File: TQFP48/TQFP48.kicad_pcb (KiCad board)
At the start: 2 copper layers, 61.2 x 18 mm, 11 parts, among them J1 Conn_01x24, J2 Conn_02x24_Counter_Clockwise, J3 Conn_02x24_Counter_Clockwise, J4 Conn_01x24, J5 Conn_01x05

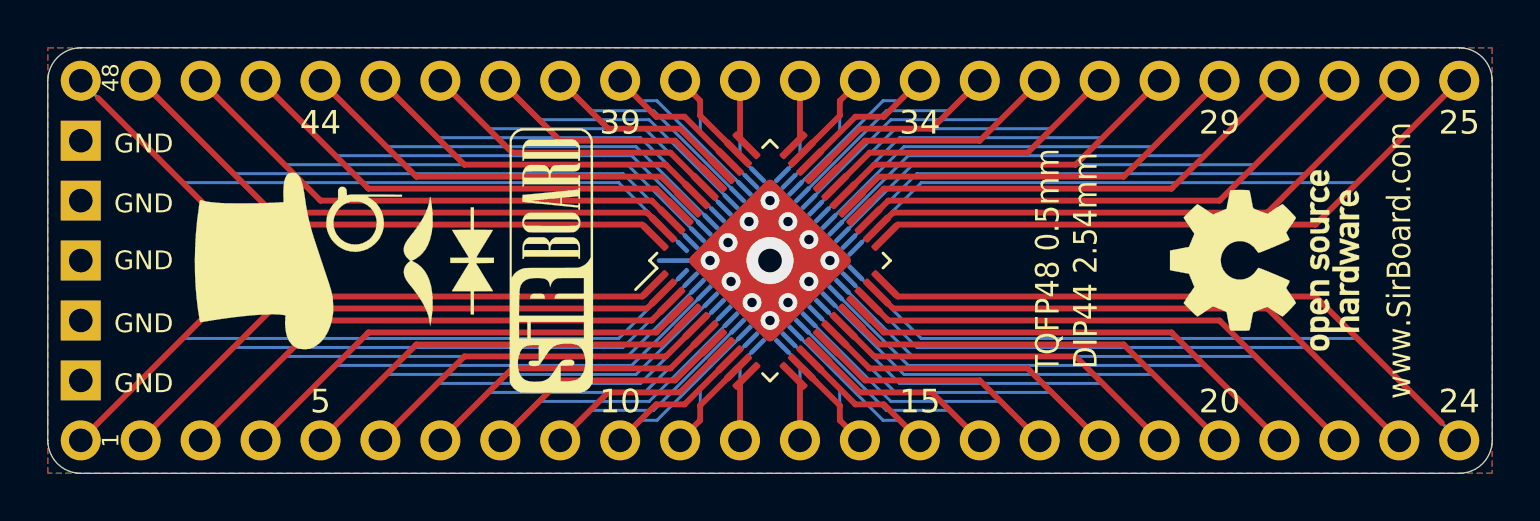
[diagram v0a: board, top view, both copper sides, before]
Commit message: Board Updates
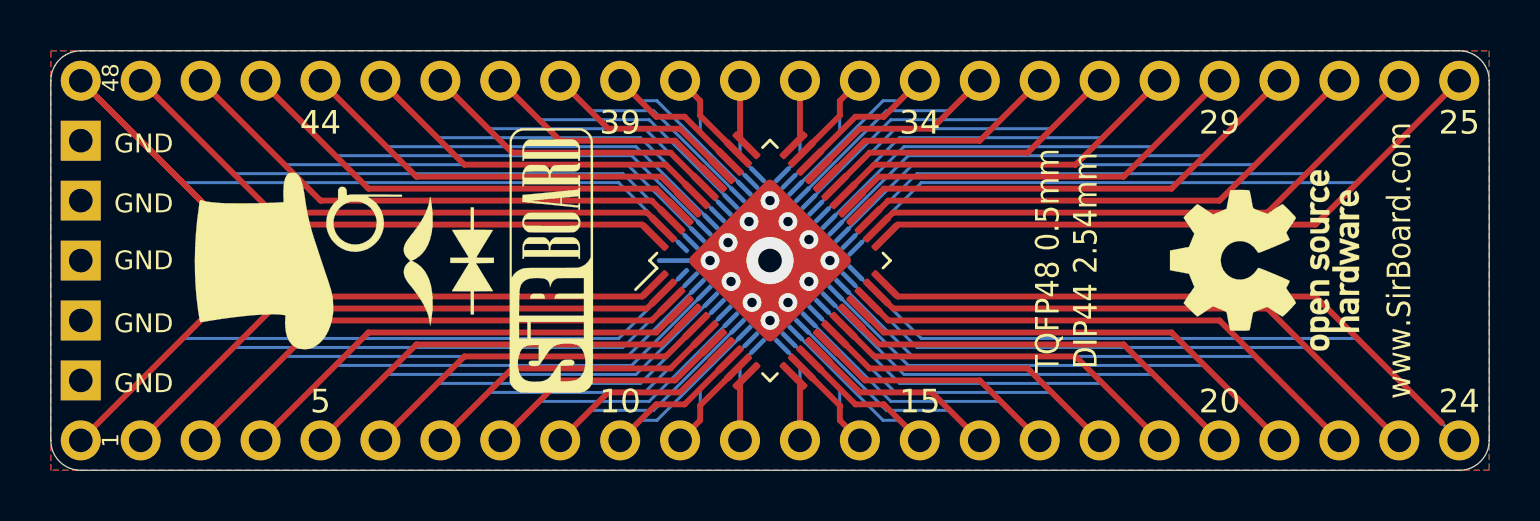
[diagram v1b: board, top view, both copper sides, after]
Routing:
- net Net-(J2-Pad48): track 54.5 -> 62.1 mm
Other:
- board size 61.2 x 18 mm -> 61 x 17.8 mm
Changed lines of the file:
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@@
     (thickness 1.6)
     (drawings 76)
-    (tracks 326)
+    (tracks 327)
     (zones 0)
     (modules 11)
@@
     (38 B.Mask user hide)
     (39 F.Mask user hide)
-    (40 Dwgs.User user)
+    (40 Dwgs.User user hide)
     (41 Cmts.User user hide)
     (42 Eco1.User user hide)
@@
       (xy 0.500964 -3.601424)) (layer F.SilkS) (width 0.01))
   )
-  (dimension 18.034 (width 0.15) (layer Dwgs.User)
-    (gr_text "18.034 mm" (at 30.196 35.56 270) (layer Dwgs.User)
+  (gr_line (start 97.917 43.18) (end 97.917 27.94) (layer Edge.Cuts) (width 0.05))
+  (gr_line (start 38.227 44.45) (end 96.647 44.45) (layer Edge.Cuts) (width 0.05))
+  (gr_line (start 36.957 27.94) (end 36.957 43.18) (layer Edge.Cuts) (width 0.05))
+  (gr_line (start 96.647 26.67) (end 38.227 26.67) (layer Edge.Cuts) (width 0.05))
+  (gr_arc (start 96.647 27.94) (end 97.917 27.94) (angle -90) (layer Edge.Cuts) (width 0.05))
+  (gr_arc (start 96.647 43.18) (end 96.647 44.45) (angle -90) (layer Edge.Cuts) (width 0.05))
+  (gr_arc (start 38.227 43.18) (end 36.957 43.18) (angle -90) (layer Edge.Cuts) (width 0.05))
+  (gr_arc (start 38.227 27.94) (end 38.227 26.67) (angle -90) (layer Edge.Cuts) (width 0.05))
+  (dimension 17.78 (width 0.15) (layer Dwgs.User)
+    (gr_text "17.780 mm" (at 30.323 35.56 270) (layer Dwgs.User)
       (effects (font (size 1 1) (thickness 0.15)) hide)
     )
-    (feature1 (pts (xy 38.227 44.577) (xy 30.909579 44.577)))
-    (feature2 (pts (xy 38.227 26.543) (xy 30.909579 26.543)))
-    (crossbar (pts (xy 31.496 26.543) (xy 31.496 44.577)))
-    (arrow1a (pts (xy 31.496 44.577) (xy 30.909579 43.450496)))
-    (arrow1b (pts (xy 31.496 44.577) (xy 32.082421 43.450496)))
-    (arrow2a (pts (xy 31.496 26.543) (xy 30.909579 27.669504)))
-    (arrow2b (pts (xy 31.496 26.543) (xy 32.082421 27.669504)))
+    (feature1 (pts (xy 38.354 44.45) (xy 31.036579 44.45)))
+    (feature2 (pts (xy 38.354 26.67) (xy 31.036579 26.67)))
+    (crossbar (pts (xy 31.623 26.67) (xy 31.623 44.45)))
+    (arrow1a (pts (xy 31.623 44.45) (xy 31.036579 43.323496)))
+    (arrow1b (pts (xy 31.623 44.45) (xy 32.209421 43.323496)))
+    (arrow2a (pts (xy 31.623 26.67) (xy 31.036579 27.796504)))
+    (arrow2b (pts (xy 31.623 26.67) (xy 32.209421 27.796504)))
   )
   (dimension 15.24 (width 0.15) (layer Dwgs.User)
@@
     (arrow2b (pts (xy 38.227 24.511) (xy 39.353504 23.924579)))
   )
-  (dimension 61.214 (width 0.15) (layer Dwgs.User)
-    (gr_text "61.214 mm" (at 67.437 20.798) (layer Dwgs.User)
+  (dimension 60.96 (width 0.15) (layer Dwgs.User)
+    (gr_text "60.960 mm" (at 67.437 20.798) (layer Dwgs.User)
       (effects (font (size 1 1) (thickness 0.15)) hide)
     )
-    (feature1 (pts (xy 98.044 27.94) (xy 98.044 21.511579)))
-    (feature2 (pts (xy 36.83 27.94) (xy 36.83 21.511579)))
-    (crossbar (pts (xy 36.83 22.098) (xy 98.044 22.098)))
-    (arrow1a (pts (xy 98.044 22.098) (xy 96.917496 22.684421)))
-    (arrow1b (pts (xy 98.044 22.098) (xy 96.917496 21.511579)))
-    (arrow2a (pts (xy 36.83 22.098) (xy 37.956504 22.684421)))
-    (arrow2b (pts (xy 36.83 22.098) (xy 37.956504 21.511579)))
+    (feature1 (pts (xy 97.917 27.94) (xy 97.917 21.511579)))
+    (feature2 (pts (xy 36.957 27.94) (xy 36.957 21.511579)))
+    (crossbar (pts (xy 36.957 22.098) (xy 97.917 22.098)))
+    (arrow1a (pts (xy 97.917 22.098) (xy 96.790496 22.684421)))
+    (arrow1b (pts (xy 97.917 22.098) (xy 96.790496 21.511579)))
+    (arrow2a (pts (xy 36.957 22.098) (xy 38.083504 22.684421)))
+    (arrow2b (pts (xy 36.957 22.098) (xy 38.083504 21.511579)))
   )
   (gr_text GND (at 40.894 30.48 180) (layer B.SilkS)
@@
     (effects (font (size 1 0.9) (thickness 0.15)))
   )
-  (gr_line (start 98.044 43.18) (end 98.044 27.94) (layer Edge.Cuts) (width 0.05))
-  (gr_line (start 38.227 44.577) (end 96.647 44.577) (layer Edge.Cuts) (width 0.05))
-  (gr_line (start 36.83 27.94) (end 36.83 43.18) (layer Edge.Cuts) (width 0.05))
-  (gr_line (start 96.647 26.543) (end 38.227 26.543) (layer Edge.Cuts) (width 0.05))
-  (gr_arc (start 96.647 27.94) (end 98.044 27.94) (angle -90) (layer Edge.Cuts) (width 0.05))
-  (gr_arc (start 96.647 43.18) (end 96.647 44.577) (angle -90) (layer Edge.Cuts) (width 0.05))
-  (gr_arc (start 38.227 43.18) (end 36.83 43.18) (angle -90) (layer Edge.Cuts) (width 0.05))
-  (gr_arc (start 38.227 27.94) (end 38.227 26.543) (angle -90) (layer Edge.Cuts) (width 0.05))
   (segment (start 72.324876 36.558788) (end 72.850088 37.084) (width 0.25) (layer F.Cu) (net 1))
   (segment (start 72.850088 37.084) (end 90.551 37.084) (width 0.25) (layer F.Cu) (net 1))
@@
   (segment (start 61.02373 32.258) (end 42.545 32.258) (width 0.127) (layer B.Cu) (net 25))
   (segment (start 42.545 32.258) (end 39.352848 29.065848) (width 0.127) (layer B.Cu) (net 25))
+  (segment (start 43.587955 33.300955) (end 38.227 27.94) (width 0.25) (layer F.Cu) (net 25))
   (segment (start 40.767 27.94) (end 46.355 33.528) (width 0.25) (layer F.Cu) (net 26))
   (segment (start 62.22302 33.528) (end 62.902678 34.207658) (width 0.25) (layer F.Cu) (net 26))
@@
     (polygon
       (pts
-        (xy 36.83 26.543) (xy 98.044 26.543) (xy 98.044 44.577) (xy 36.83 44.577)
+        (xy 36.957 26.67) (xy 97.917 26.67) (xy 97.917 44.45) (xy 36.957 44.45)
       )
     )
@@
     (polygon
       (pts
-        (xy 36.83 26.543) (xy 98.044 26.543) (xy 98.044 44.577) (xy 36.83 44.577)
+        (xy 36.957 26.67) (xy 97.917 26.67) (xy 97.917 44.45) (xy 36.957 44.45)
       )
     )
